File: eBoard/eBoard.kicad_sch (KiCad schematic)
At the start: 90 parts, among them Q10 PN2222A, Q11 PN2222A, Q12 PN2222A, Q9 PN2222A, U11 74HC595, U12 74HC595, U2 74HC595, U68 DRV5055A3xLPGxQ1, U69 DRV5055A3xLPGxQ1, U70 DRV5055A3xLPGxQ1, U71 DRV5055A3xLPGxQ1

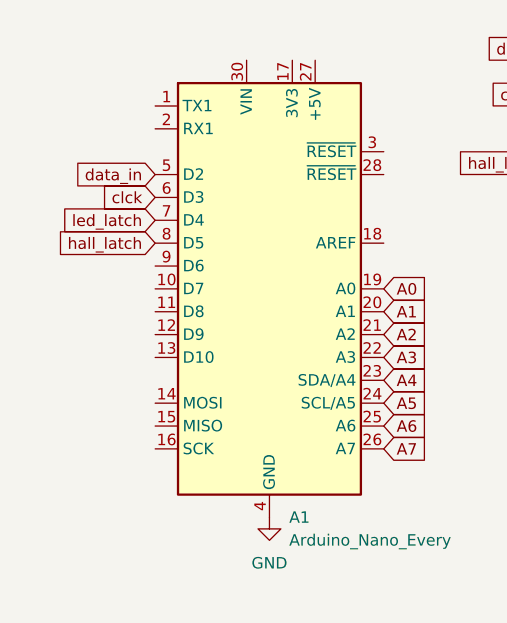
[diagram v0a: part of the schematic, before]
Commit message: spi working
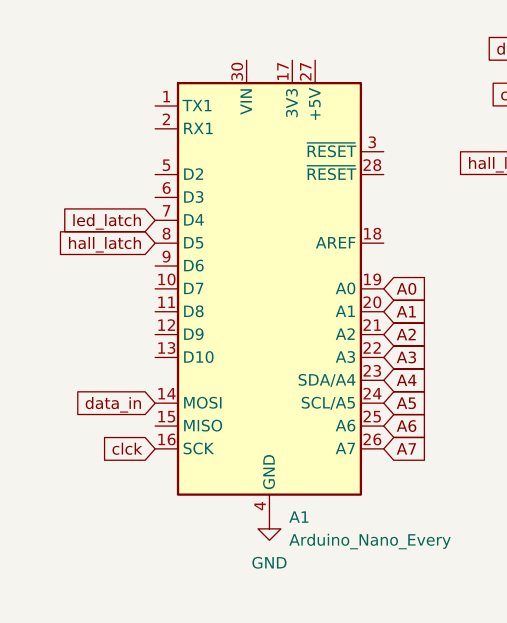
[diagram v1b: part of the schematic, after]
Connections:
- net clck: now also A1.16 (SCK); no longer A1.6 (D3)
- net data_in: now also A1.14 (MOSI); no longer A1.5 (D2)
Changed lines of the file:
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@@
     )
   )
-  (global_label "data_in" (shape input) (at 38.1 93.98 180) (fields_autoplaced)
+  (global_label "data_in" (shape input) (at 38.1 119.38 180) (fields_autoplaced)
     (effects (font (size 1.27 1.27)) (justify right))
-    (property "Intersheetrefs" "${INTERSHEET_REFS}" (at 28.2207 93.98 0)
+    (property "Intersheetrefs" "${INTERSHEET_REFS}" (at 28.2207 119.38 0)
       (effects (font (size 1.27 1.27)) (justify right) hide)
     )
@@
     (effects (font (size 1.27 1.27)) (justify right))
     (property "Intersheetrefs" "${INTERSHEET_REFS}" (at 83.919 176.53 0)
+      (effects (font (size 1.27 1.27)) (justify right) hide)
+    )
+  )
+  (global_label "clck" (shape input) (at 38.1 124.46 180) (fields_autoplaced)
+    (effects (font (size 1.27 1.27)) (justify right))
+    (property "Intersheetrefs" "${INTERSHEET_REFS}" (at 31.2443 124.46 0)
       (effects (font (size 1.27 1.27)) (justify right) hide)
     )
@@
       (effects (font (size 1.27 1.27)) (justify right) hide)
     )
-  )
-  (global_label "clck" (shape input) (at 38.1 96.52 180) (fields_autoplaced)
-    (effects (font (size 1.27 1.27)) (justify right))
-    (property "Intersheetrefs" "${INTERSHEET_REFS}" (at 31.2443 96.52 0)
-      (effects (font (size 1.27 1.27)) (justify right) hide)
-    )
